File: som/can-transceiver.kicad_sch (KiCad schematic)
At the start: 10 parts, among them U2 TCAN844DRBRQ1, U3 TS5A3166YZPR

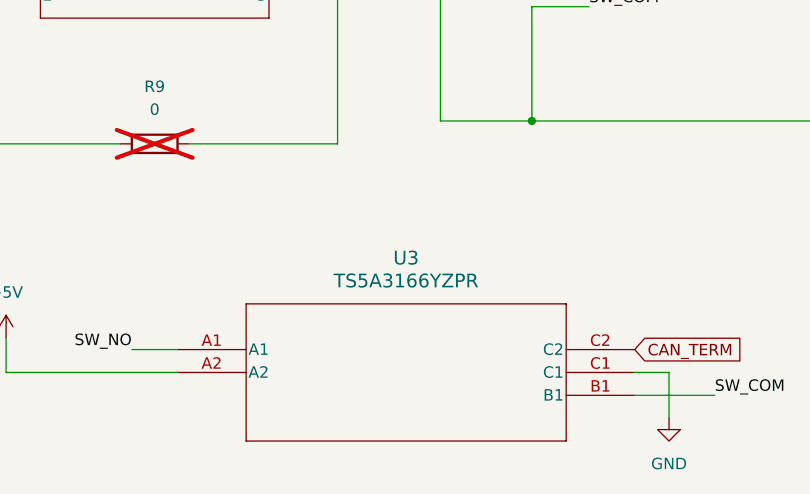
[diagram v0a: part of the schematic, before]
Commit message: First proto hardware
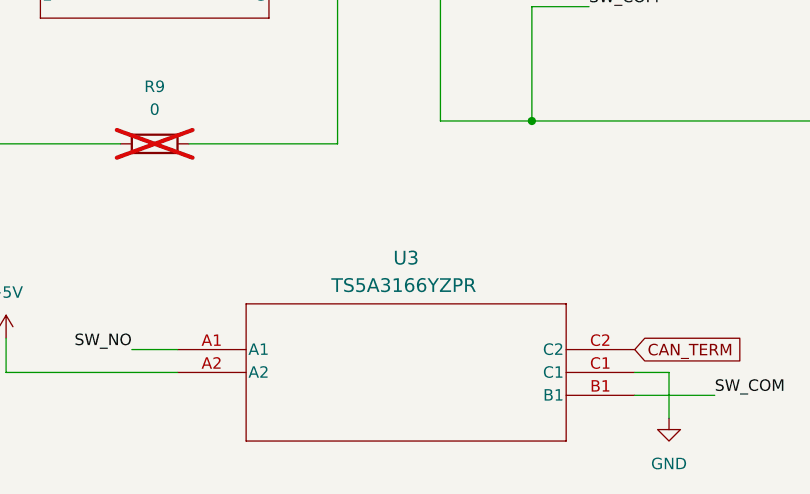
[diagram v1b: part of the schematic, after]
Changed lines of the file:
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@@
 		(in_pos_files yes)
 		(dnp no)
-		(fields_autoplaced yes)
 		(property "Reference" "U3"
 			(at 173.99 130.81 0)
@@
 		)
 		(property "Value" "TS5A3166YZPR"
-			(at 173.99 133.35 0)
+			(at 173.736 133.858 0)
 			(show_name no)
 			(do_not_autoplace no)
